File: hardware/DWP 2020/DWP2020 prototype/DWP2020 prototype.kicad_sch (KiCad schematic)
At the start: 2 parts, among them U1 Teensy4.0, U2 SSD1351_128X128_LCD-bGeigieNa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

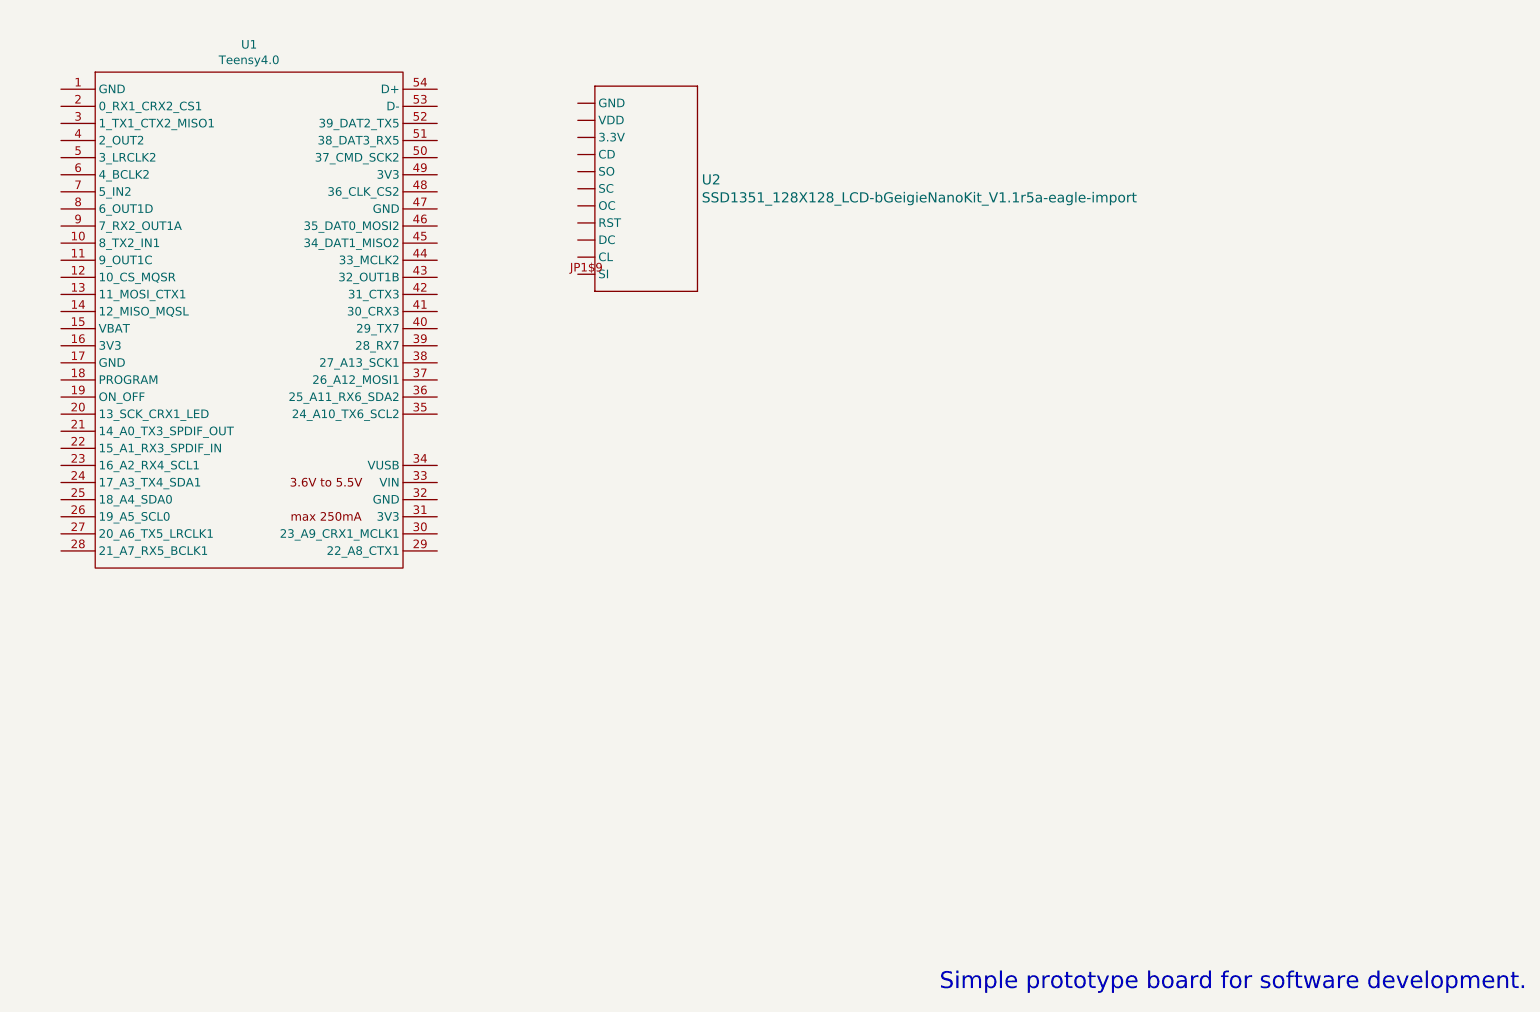
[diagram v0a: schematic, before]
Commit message: fix some typoos
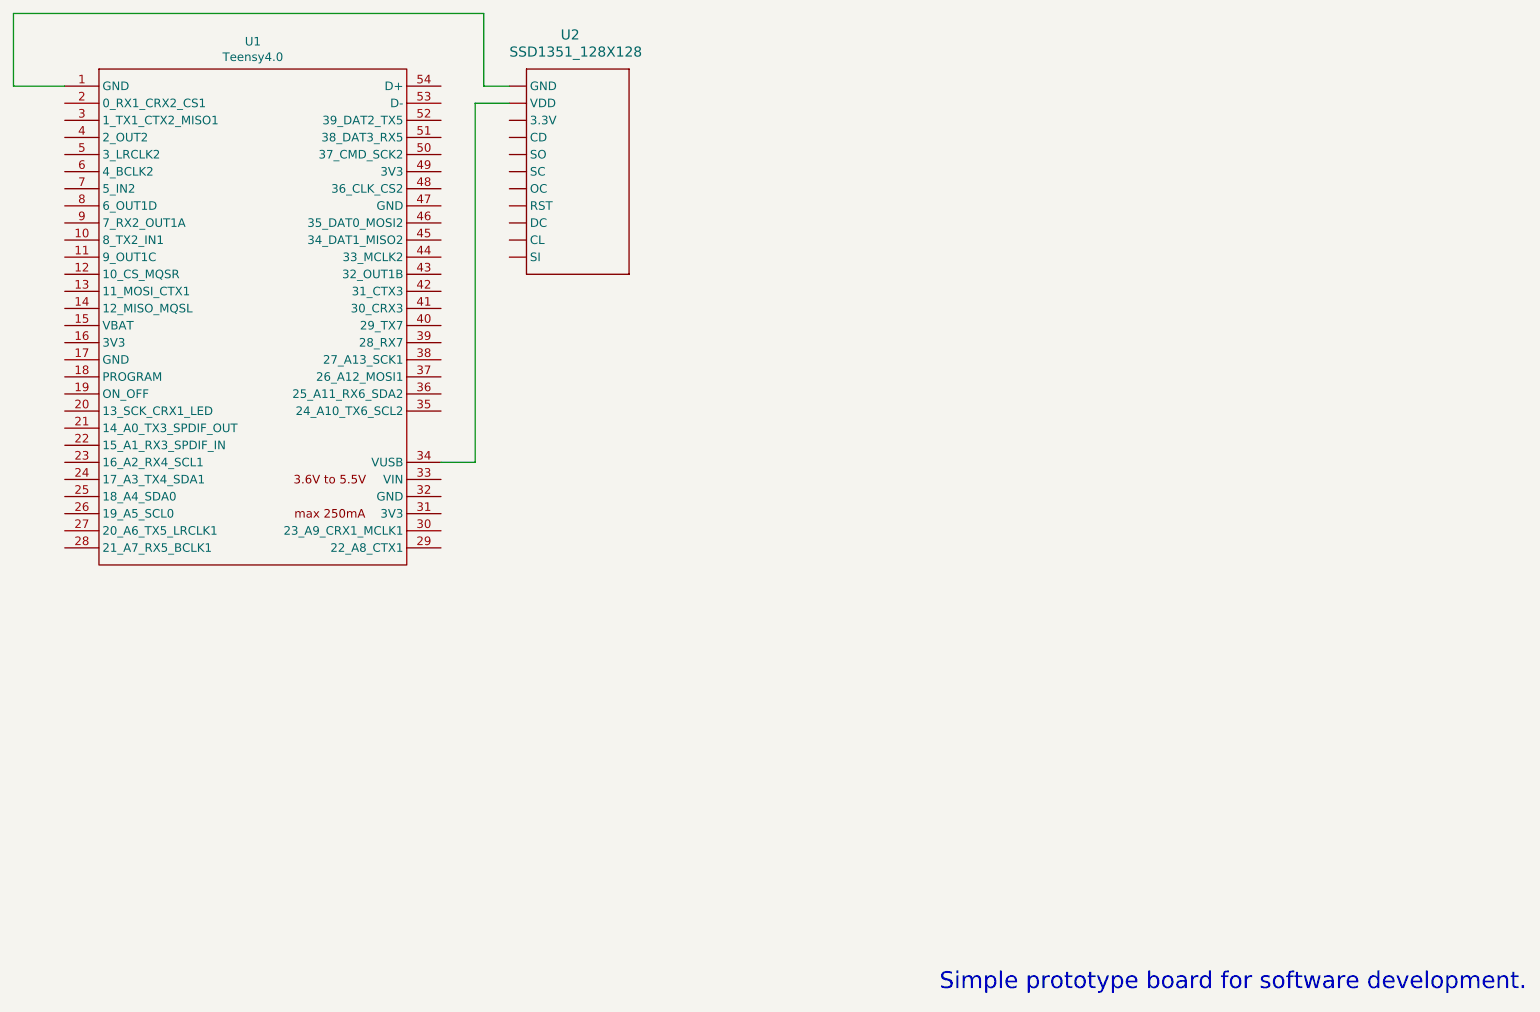
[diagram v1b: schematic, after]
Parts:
- removed U2: SSD1351_128X128_LCD-bGeigieNanoKit_V1.1r5a-eagle-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, DWP2020 prototype:SSD1351_128X128_LCD, symbol import_from_eagle-rescue:SSD1351_128X128_LCD-bGeigieNanoKit_V1.1r5a-eagle-import
- added U2: SSD1351_128X128, DWP2020 prototype:SSD1351_128X128_LCD, symbol import_from_eagle-rescue:SSD1351_128X128
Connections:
- net at U1.1 (GND): now also U2.JP1$8 (GND)
- net at U1.34 (VUSB): now also U2.JP1$7 (VDD)
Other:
- moved on the sheet: U1
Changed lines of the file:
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@@
-(kicad_sch (version 20200608) (host eeschema "5.99.0-unknown-0bfe413~88~ubuntu18.04.1")
+(kicad_sch (version 20200608) (host eeschema "5.99.0-unknown-08c61e6~88~ubuntu18.04.1")
   (page 1 1)
   (paper "A4")
@@
     (date "2020-06-17")
   )
+  (wire (pts (xy 49.53 27.305) (xy 49.53 38.1))
+    (stroke (width 0) (type solid) (color 0 0 0 0))
+  )
+  (wire (pts (xy 49.53 38.1) (xy 57.15 38.1))
+    (stroke (width 0) (type solid) (color 0 0 0 0))
+  )
+  (wire (pts (xy 113.03 93.98) (xy 118.11 93.98))
+    (stroke (width 0) (type solid) (color 0 0 0 0))
+  )
+  (wire (pts (xy 118.11 40.64) (xy 123.19 40.64))
+    (stroke (width 0) (type solid) (color 0 0 0 0))
+  )
+  (wire (pts (xy 118.11 93.98) (xy 118.11 40.64))
+    (stroke (width 0) (type solid) (color 0 0 0 0))
+  )
+  (wire (pts (xy 119.38 27.305) (xy 49.53 27.305))
+    (stroke (width 0) (type solid) (color 0 0 0 0))
+  )
+  (wire (pts (xy 119.38 38.1) (xy 119.38 27.305))
+    (stroke (width 0) (type solid) (color 0 0 0 0))
+  )
+  (wire (pts (xy 119.38 38.1) (xy 123.19 38.1))
+    (stroke (width 0) (type solid) (color 0 0 0 0))
+  )
   (text "Simple prototype board for software development." (at 274.2692 172.6184 180)
     (effects (font (size 2.5 2.5)) (justify right bottom))
   )
-  (symbol (lib_id "import_from_eagle-rescue:SSD1351_128X128_LCD-bGeigieNanoKit_V1.1r5a-eagle-import") (at 148.59 58.42 0) (unit 1)
+  (symbol (lib_id "import_from_eagle-rescue:SSD1351_128X128") (at 138.43 55.88 0) (unit 1)
     (in_bom yes) (on_board yes)
-    (property "Reference" "U2" (id 0) (at 151.7651 52.0066 0)
+    (property "Reference" "U2" (id 0) (at 130.81 30.48 0)
       (effects (font (size 1.4986 1.4986)) (justify left))
     )
-    (property "Value" "SSD1351_128X128_LCD-bGeigieNanoKit_V1.1r5a-eagle-import" (id 1) (at 151.7651 54.6733 0)
-      (effects (font (size 1.4986 1.4986)) (justify left))
+    (property "Value" "SSD1351_128X128" (id 1) (at 123.19 33.02 0)
+      (effects (font (size 1.499 1.499)) (justify left))
     )
-    (property "Footprint" "DWP2020 prototype:SSD1351_128X128_LCD" (id 2) (at 148.59 58.42 0)
+    (property "Footprint" "DWP2020 prototype:SSD1351_128X128_LCD" (id 2) (at 138.4296 55.8802 0)
       (effects (font (size 1.27 1.27)) hide)
     )
-    (property "Datasheet" "" (id 3) (at 148.59 58.42 0)
+    (property "Datasheet" "" (id 3) (at 138.43 55.88 0)
       (effects (font (size 1.27 1.27)) hide)
     )
   )
-  (symbol (lib_id "Teensy4:Teensy4.0") (at 84.5312 72.8472 0) (unit 1)
+  (symbol (lib_id "Teensy4:Teensy4.0") (at 85.09 72.39 0) (unit 1)
     (in_bom yes) (on_board yes)
-    (property "Reference" "U1" (id 0) (at 84.5312 31.934 0))
-    (property "Value" "Teensy4.0" (id 1) (at 84.5312 34.2327 0))
-    (property "Footprint" "Teensy:Teensy40" (id 2) (at 74.371 67.7674 0)
+    (property "Reference" "U1" (id 0) (at 85.09 31.4768 0))
+    (property "Value" "Teensy4.0" (id 1) (at 85.09 33.7755 0))
+    (property "Footprint" "Teensy:Teensy40" (id 2) (at 74.9298 67.3102 0)
       (effects (font (size 1.27 1.27)) hide)
     )
-    (property "Datasheet" "" (id 3) (at 74.3712 67.7672 0)
+    (property "Datasheet" "" (id 3) (at 74.93 67.31 0)
       (effects (font (size 1.27 1.27)) hide)
     )
@@
       (reference "U1") (unit 1)
     )
-    (path "/620b6ebe-1873-4600-987b-50cce9a7f2c9"
+    (path "/c2fe866b-0538-436e-a065-5c65dd070b82"
       (reference "U2") (unit 1)
     )
